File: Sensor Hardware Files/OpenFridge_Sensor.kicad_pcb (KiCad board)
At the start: 2 copper layers, 3 parts, among them U1 TMP101, U2 STM32F103C8Tx, U3 BH1730FVC

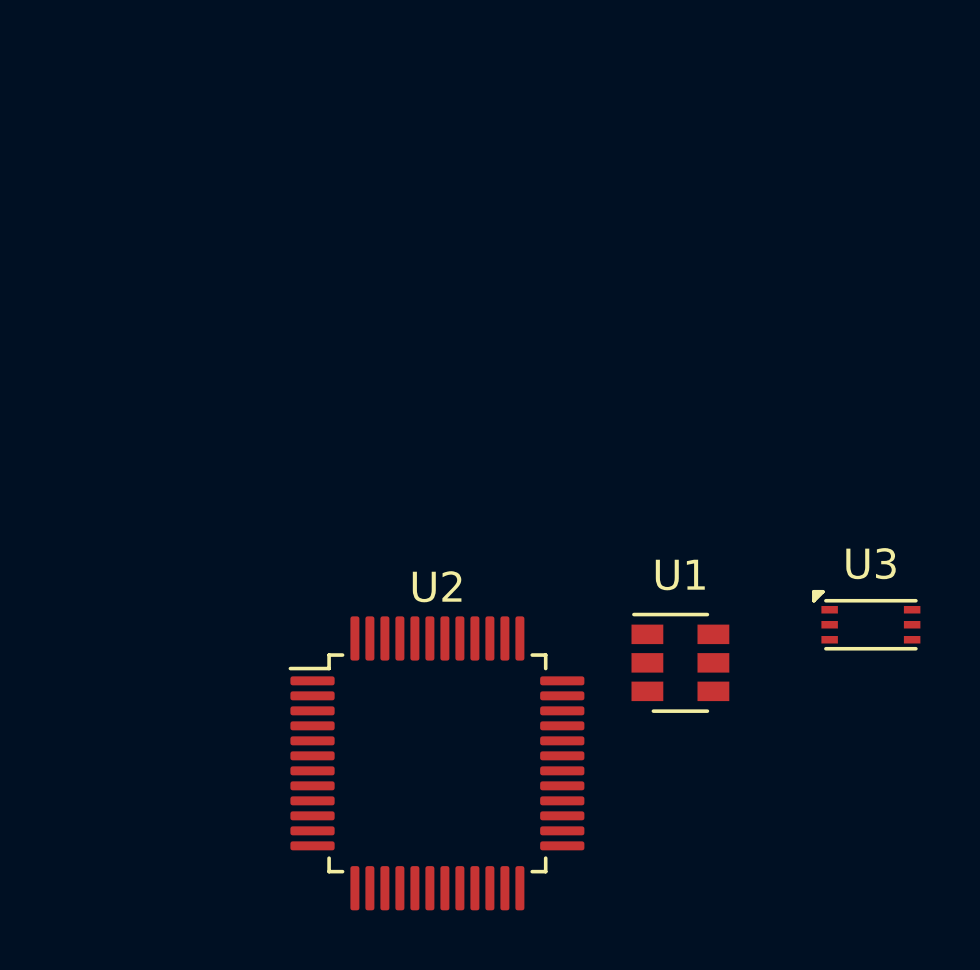
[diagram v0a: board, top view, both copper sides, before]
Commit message: update footprints
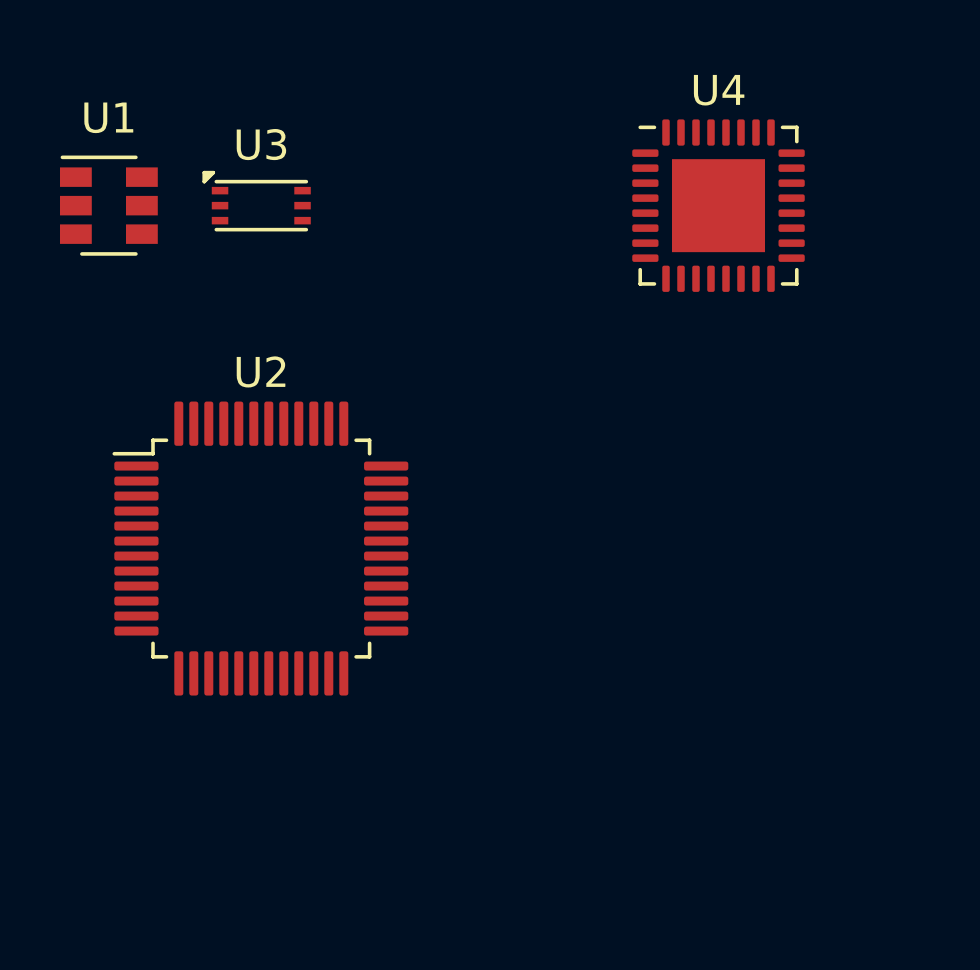
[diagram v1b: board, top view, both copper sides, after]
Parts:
- added U4: AT86RF231-ZU, Package_DFN_QFN:VQFN-32-1EP_5x5mm_P0.5mm_EP3.1x3.1mm, F.Cu at (142.2, 72.4)
- moved U3 24.7 mm to (127.0, 72.4)
- moved U1 24.4 mm to (121.9, 72.4)
- moved U2 9.26 mm to (127.0, 83.8)
